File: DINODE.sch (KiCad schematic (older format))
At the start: 35 parts, among them J1 Barrel_Jack, J10 Conn_01x03_Male, J11 Conn_02x04_Odd_Even, J12 Conn_01x03_Female, J13 Conn_02x04_Odd_Even, J2 Conn_01x02_Male, J3 Conn_01x07, J4 Conn_01x16, J5 Conn_02x04_Odd_Even, J6 Conn_02x04_Odd_Even, J7 Conn_02x04_Odd_Even, J8 AVR-ISP-6, J9 Conn_02x04_Odd_Even, SW1 SW_Push, U1 L7805, U2 ATmega32-16AU, U3 LM1117-3.3, Y1 16MHz

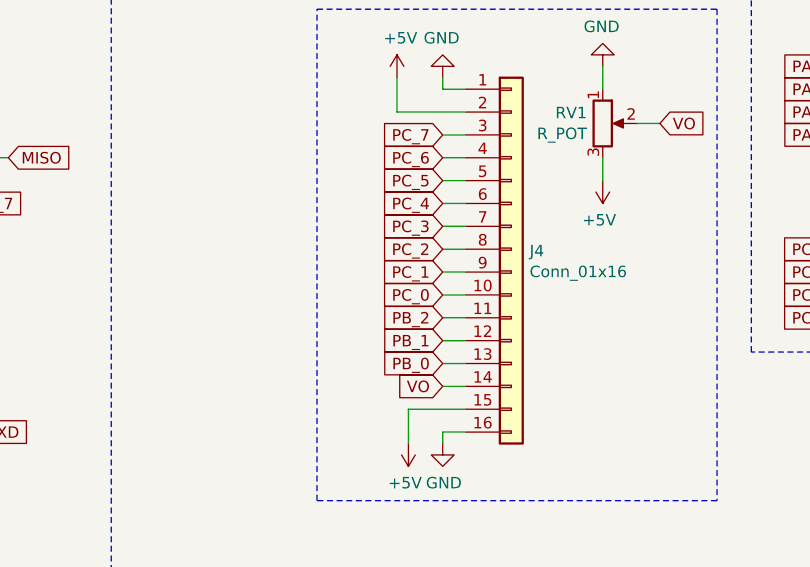
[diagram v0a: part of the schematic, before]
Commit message: updated gerber files
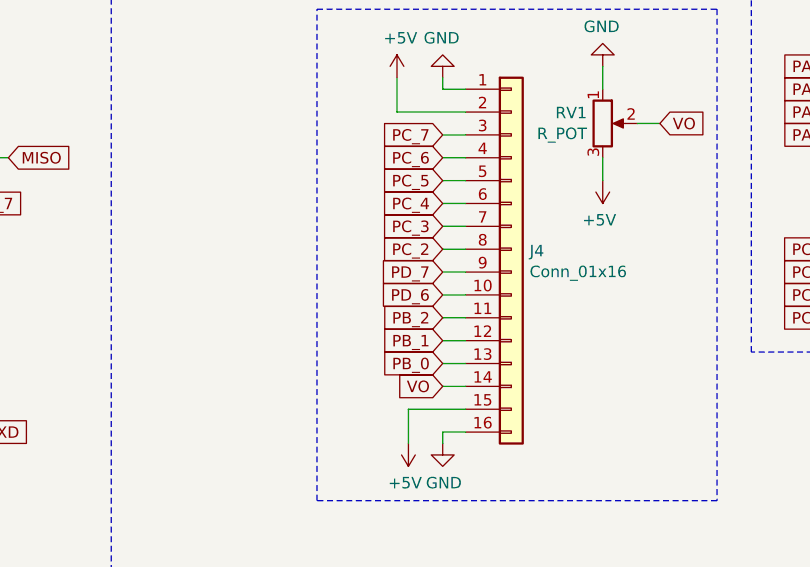
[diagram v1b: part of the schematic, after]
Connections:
- net PC_0: no longer J4.10 (Pin_10)
- net PC_1: no longer J4.9 (Pin_9)
- net PD_6: now also J4.10 (Pin_10)
- net PD_7: now also J4.9 (Pin_9)
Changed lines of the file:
@@
 PC_2
 Text GLabel 6300 4750 0    50   Input ~ 0
-PC_1
+PD_7
 Text GLabel 6300 4850 0    50   Input ~ 0
-PC_0
+PD_6
 Text GLabel 6300 4950 0    50   Input ~ 0
 PB_2
